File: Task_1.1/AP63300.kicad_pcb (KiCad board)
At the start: 2 copper layers, 30 x 30 mm, 14 parts, among them J1 Conn_01x03, U1 AP63300

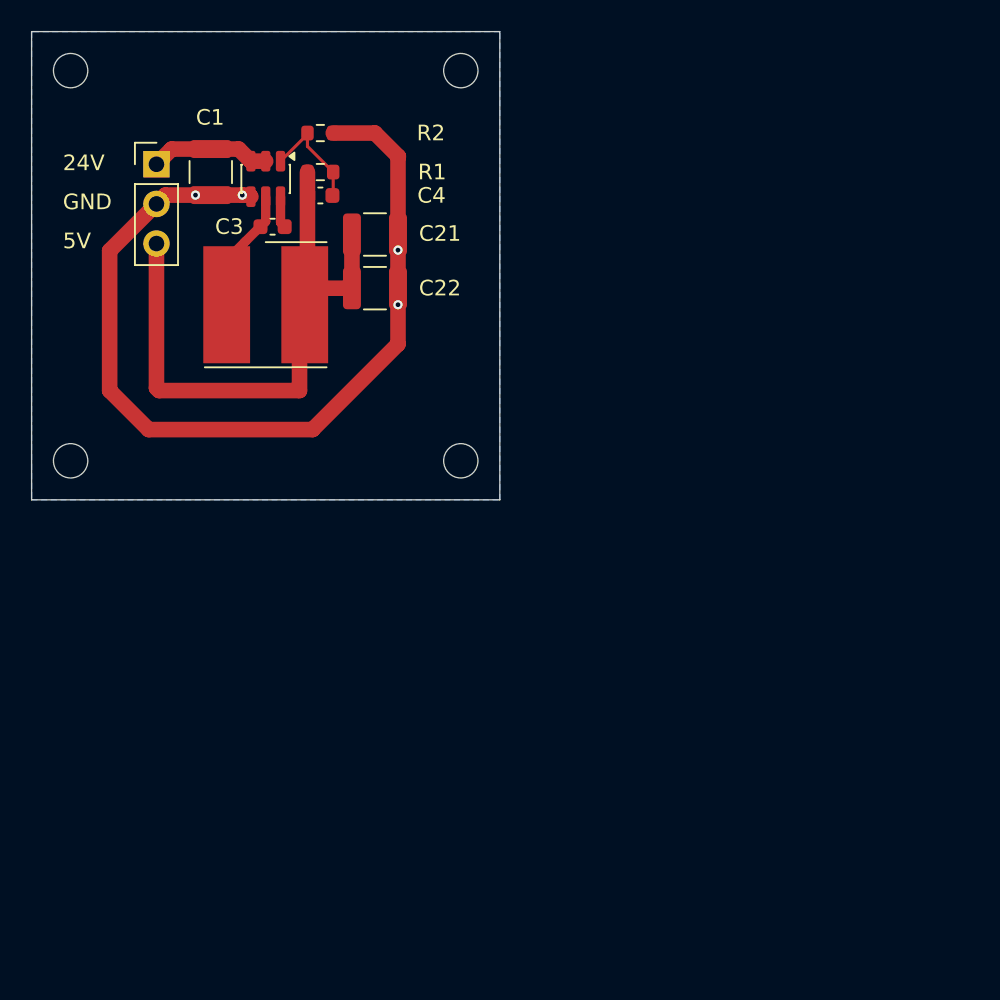
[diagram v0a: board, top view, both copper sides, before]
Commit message: Uploaded pics for the pdf report
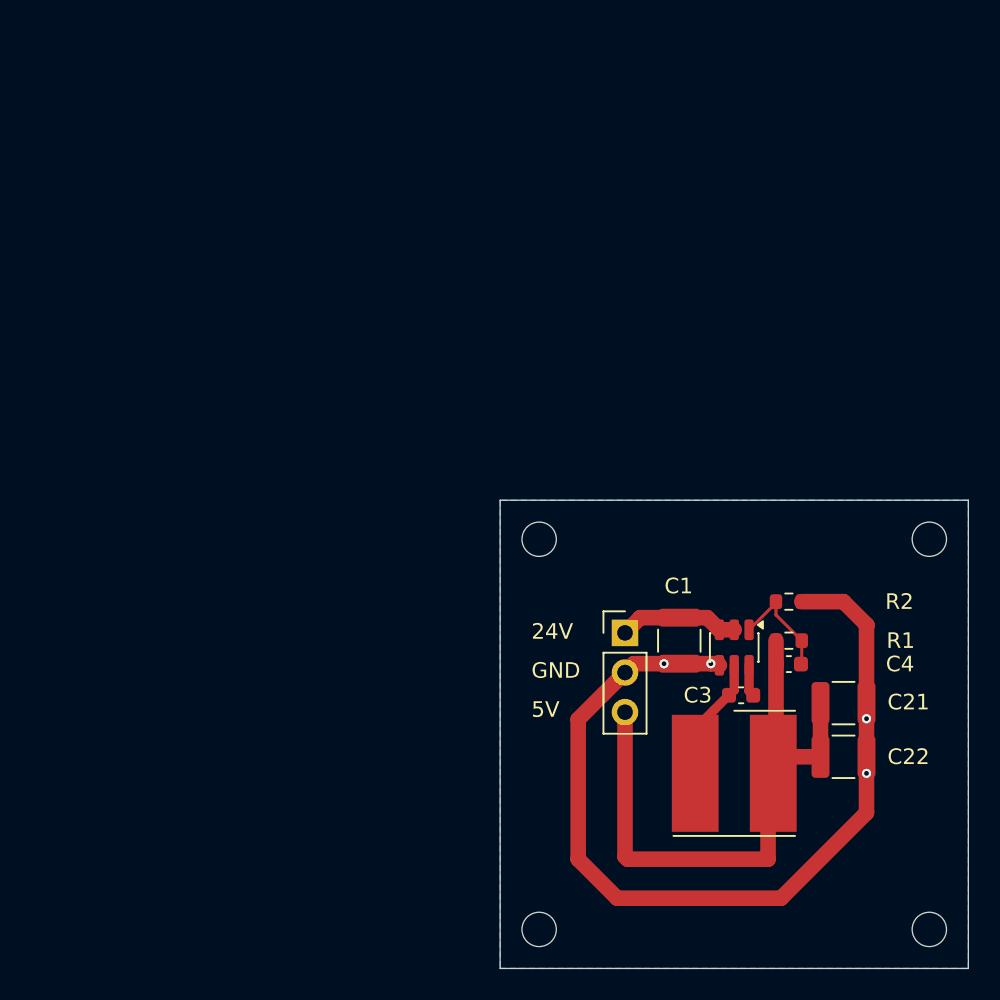
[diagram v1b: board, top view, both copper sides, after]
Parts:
- moved C1 42.5 mm to (61.5, 59.0)
- moved C22 42.5 mm to (72.0, 66.5)
- moved J1 42.5 mm to (58.0, 58.5)
- moved L1 42.5 mm to (65.0, 67.5)
- moved REF** 42.5 mm to (52.5, 77.5)
- moved REF** 42.5 mm to (52.5, 52.5)
- moved REF** 42.5 mm to (77.5, 77.5)
- moved U1 42.5 mm to (65.0, 59.5)
- moved C21 42.5 mm to (72.0, 63.0)
- moved C3 42.5 mm to (65.5, 62.5)
- moved C4 42.5 mm to (68.5, 60.5)
- moved R1 42.5 mm to (68.5, 59.0)
- moved R2 42.5 mm to (68.5, 56.5)
- moved REF** 42.5 mm to (77.5, 52.5)
